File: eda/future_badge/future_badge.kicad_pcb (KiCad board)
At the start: 2 copper layers, 137.1 x 80 mm, 6 parts

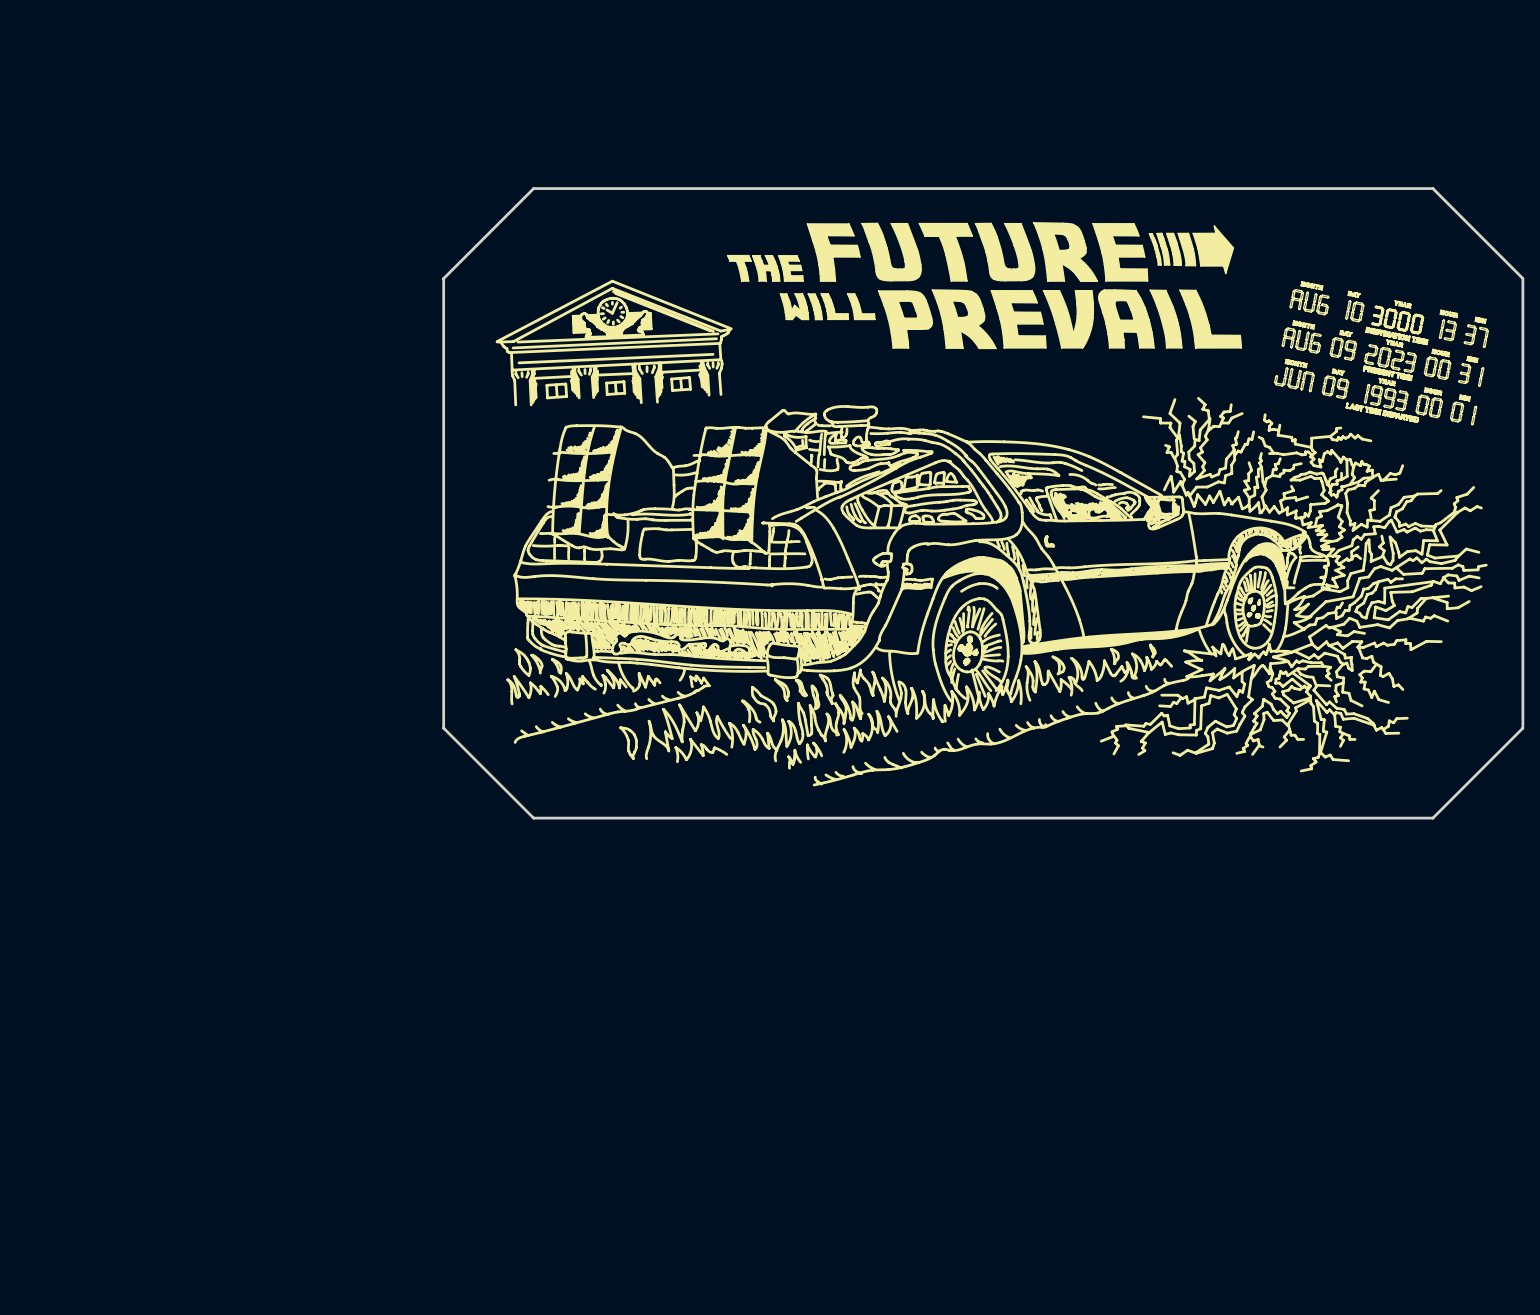
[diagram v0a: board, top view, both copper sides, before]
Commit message: PCB layout
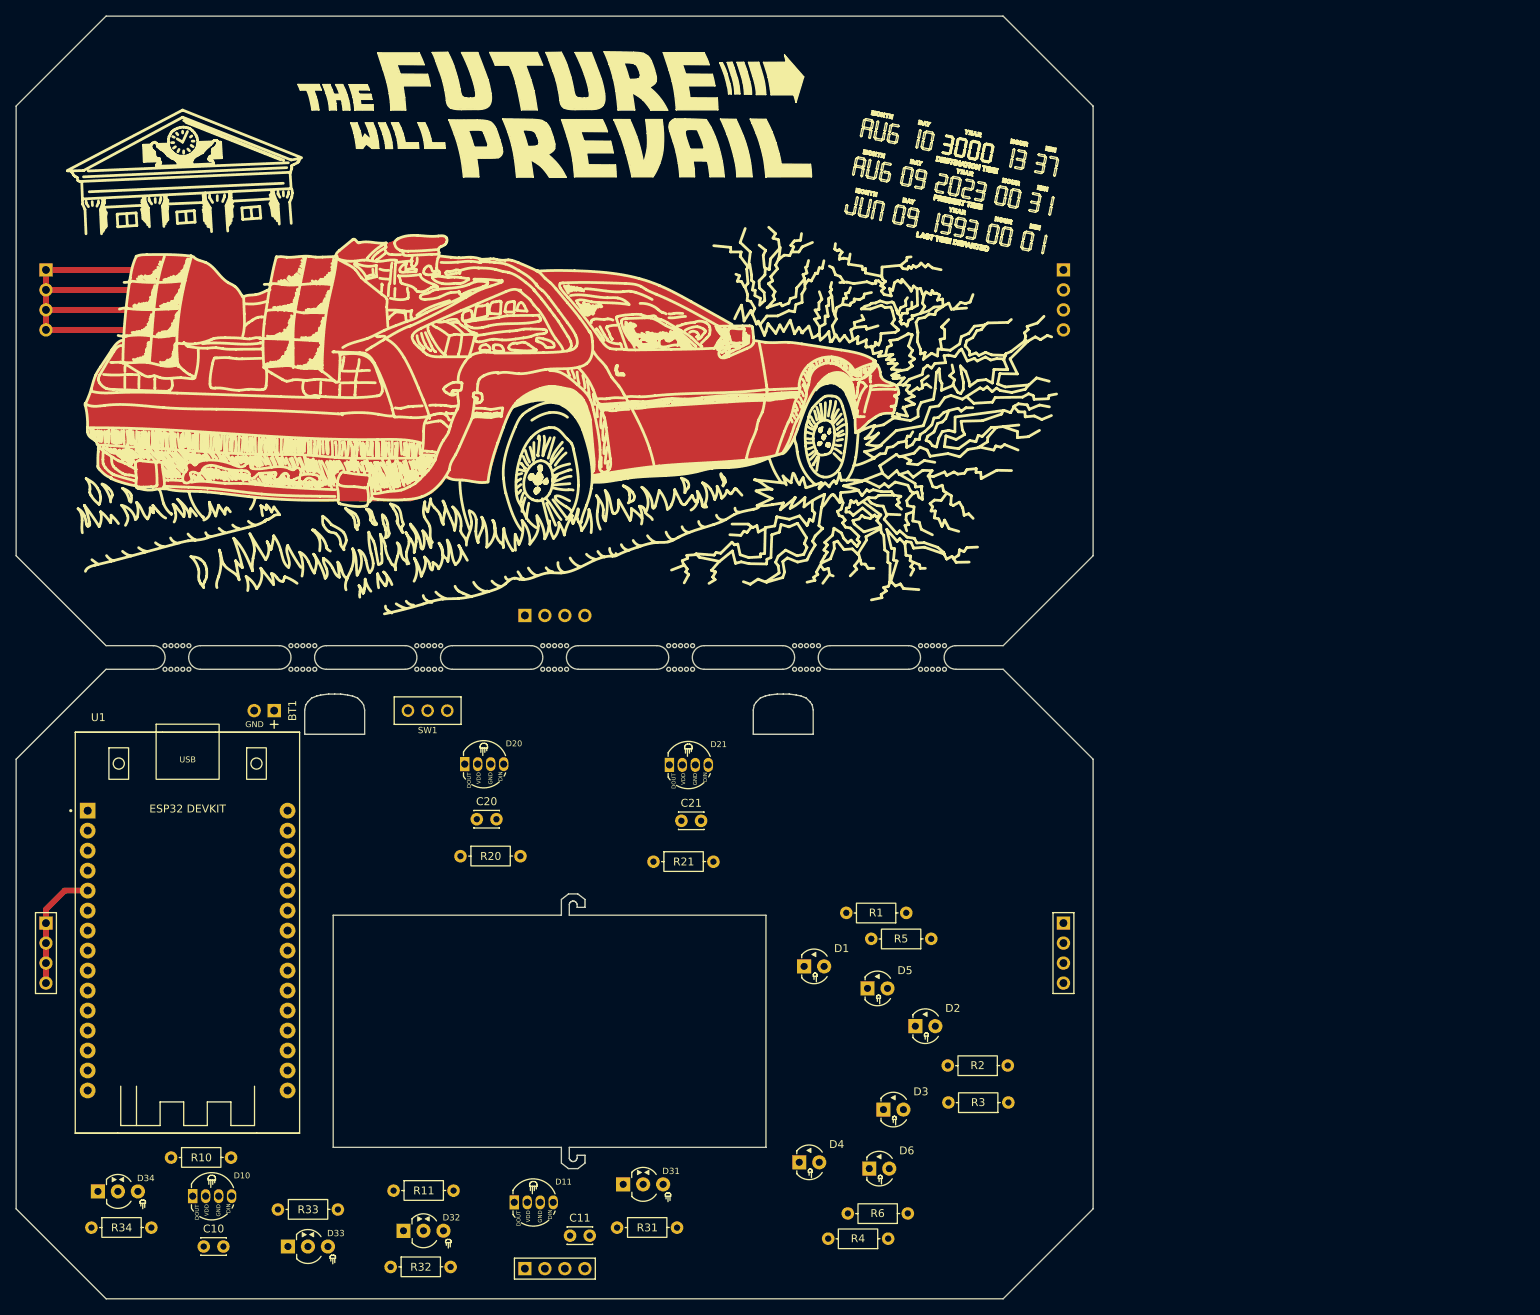
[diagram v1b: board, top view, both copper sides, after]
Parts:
- added BT1: Battery_9V, 0_local:Battery_Lead_Wire_Connector, F.Cu at (52.5, 106.0)
- added C10: 100nF, 0_local:C_Disc_D3.0mm_W2.0mm_P2.50mm, F.Cu at (43.5, 174.1)
- added C11: 100nF, 0_local:C_Disc_D3.0mm_W2.0mm_P2.50mm, F.Cu at (90.1, 172.7)
- added C20: 100nF, 0_local:C_Disc_D3.0mm_W2.0mm_P2.50mm, F.Cu at (78.2, 119.8)
- added C21: 100nF, 0_local:C_Disc_D3.0mm_W2.0mm_P2.50mm, F.Cu at (104.2, 120.0)
- added D1: LED_3mm, 0_local:LED_D3.0mm-2, F.Cu at (119.8, 138.5)
- added D10: LED_WS2812D_5mm, 0_local:LED_D5.0mm-4_WS2812D_front_new, F.Cu at (42.6, 167.7)
- added D11: LED_WS2812D_5mm, 0_local:LED_D5.0mm-4_WS2812D_front_new, F.Cu at (83.5, 168.5)
- added D2: LED_3mm, 0_local:LED_D3.0mm-2, F.Cu at (134.0, 146.1)
- added D20: LED_WS2812D_5mm, 0_local:LED_D5.0mm-4_WS2812D_front_new, F.Cu at (77.2, 112.8)
- added D21: LED_WS2812D_5mm, 0_local:LED_D5.0mm-4_WS2812D_front_new, F.Cu at (103.2, 112.9)
- added D3: LED_3mm, 0_local:LED_D3.0mm-2, F.Cu at (129.9, 156.7)
- added D31: YEL_RED_CC_3mm, 0_local:LED_D3.0mm-3-TwoColor, F.Cu at (96.8, 166.2)
- added D32: YEL_RED_CC_3mm, 0_local:LED_D3.0mm-3-TwoColor, F.Cu at (68.9, 172.1)
- added D33: YEL_RED_CC_3mm, 0_local:LED_D3.0mm-3-TwoColor, F.Cu at (54.2, 174.1)
- added D34: YEL_RED_CC_3mm, 0_local:LED_D3.0mm-3-TwoColor, F.Cu at (30.1, 167.1)
- added D4: LED_3mm, 0_local:LED_D3.0mm-2, F.Cu at (119.2, 163.4)
- added D5: LED_3mm, 0_local:LED_D3.0mm-2, F.Cu at (127.9, 141.3)
- added D6: LED_3mm, 0_local:LED_D3.0mm-2, F.Cu at (128.1, 164.2)
- added G***: 3000_Society_Logo_Back_2500dpi, 0_org_logos:3000_Society_Logo_Back_2500dpi, F.Cu at (65.5, 115.5)
- added G***: DHA_Logo_Back_1500dpi, 0_org_logos:DHA_Logo_Back_1500dpi, F.Cu at (134.0, 117.0)
- added G***: LOGO, 0_alt_bier:logo-alt_bier-500dpi-18x45mm-back, F.Cu at (41.5, 136.0)
- added G***: LOGO, 0_org_logos:DC214_Logo_v2_Back_1200dpi, F.Cu at (92.0, 112.0)
- added R1: 47R_6.3mm, 0_local:R_Axial_DIN0207_L6.3mm_D2.5mm_P7.62mm_Horizontal, F.Cu at (132.8, 131.7)
- added R10: 47R_6.3mm, 0_local:R_Axial_DIN0207_L6.3mm_D2.5mm_P7.62mm_Horizontal, F.Cu at (39.4, 162.8)
- added R11: 47R_6.3mm, 0_local:R_Axial_DIN0207_L6.3mm_D2.5mm_P7.62mm_Horizontal, F.Cu at (67.7, 167.0)
- added R2: 47R_6.3mm, 0_local:R_Axial_DIN0207_L6.3mm_D2.5mm_P7.62mm_Horizontal, F.Cu at (145.7, 151.1)
- added R20: 47R_6.3mm, 0_local:R_Axial_DIN0207_L6.3mm_D2.5mm_P7.62mm_Horizontal, F.Cu at (76.2, 124.5)
- added R21: 47R_6.3mm, 0_local:R_Axial_DIN0207_L6.3mm_D2.5mm_P7.62mm_Horizontal, F.Cu at (100.7, 125.2)
- added R3: 47R_6.3mm, 0_local:R_Axial_DIN0207_L6.3mm_D2.5mm_P7.62mm_Horizontal, F.Cu at (145.8, 155.8)
- added R31: 47R_6.3mm, 0_local:R_Axial_DIN0207_L6.3mm_D2.5mm_P7.62mm_Horizontal, F.Cu at (96.1, 171.7)
- added R32: 47R_6.3mm, 0_local:R_Axial_DIN0207_L6.3mm_D2.5mm_P7.62mm_Horizontal, F.Cu at (67.3, 176.7)
- added R33: 47R_6.3mm, 0_local:R_Axial_DIN0207_L6.3mm_D2.5mm_P7.62mm_Horizontal, F.Cu at (53.0, 169.4)
- added R34: 47R_6.3mm, 0_local:R_Axial_DIN0207_L6.3mm_D2.5mm_P7.62mm_Horizontal, F.Cu at (29.3, 171.7)
- added R4: 47R_6.3mm, 0_local:R_Axial_DIN0207_L6.3mm_D2.5mm_P7.62mm_Horizontal, F.Cu at (130.5, 173.1)
- added R5: 47R_6.3mm, 0_local:R_Axial_DIN0207_L6.3mm_D2.5mm_P7.62mm_Horizontal, F.Cu at (136.0, 135.0)
- added R6: 47R_6.3mm, 0_local:R_Axial_DIN0207_L6.3mm_D2.5mm_P7.62mm_Horizontal, F.Cu at (133.0, 169.9)
- added REF**: Conn_Pin_Header_Male_Vert_Front_1x04_Pitch2.54mm, 0_local:Conn_Pin_Header_Male_Vert_Front_1x04_Pitch2.54mm, F.Cu at (84.4, 176.9)
- added REF**: future_badge_userdrawing_title, 0_local:future_badge_userdrawing_title, F.Cu at (89.3, 129.1)
- added REF**: future_badge_frontcopper_delorean, 0_local:future_badge_frontcopper_delorean, F.Cu at (85.9, 59.5)
- added REF**: Battery_9V_silk_back, 0_local:Battery_9V_silk_back, F.Cu at (88.2, 63.7)
- added REF**: Conn_Pin_Header_Female_Vert_Back_1x04_Pitch2.54mm, 0_local:Conn_Pin_Header_Female_Vert_Back_1x04_Pitch2.54mm, F.Cu at (152.8, 50.0)
- added REF**: future_badge_userdrawing_flames, 0_local:future_badge_userdrawing_flames, F.Cu at (85.8, 138.2)
- added REF**: future_badge_frontmask_delorean, 0_local:future_badge_frontmask_delorean, F.Cu at (91.9, 54.4)
- added REF**: ESP32_DEVKIT_V1_silk_back, 0_local:ESP32_DEVKIT_V1_silk_back, F.Cu at (41.5, 51.2)
- added REF**: Conn_Pin_Header_Male_Vert_Front_1x04_Pitch2.54mm, 0_local:Conn_Pin_Header_Male_Vert_Front_1x04_Pitch2.54mm, F.Cu at (152.8, 133.0)
- added REF**: future_badge_backmask_flames, 0_local:future_badge_backmask_flames, F.Cu at (87.1, 52.4)
- added REF**: Conn_Pin_Header_Female_Vert_Back_1x04_Pitch2.54mm, 0_local:Conn_Pin_Header_Female_Vert_Back_1x04_Pitch2.54mm, F.Cu at (84.4, 93.9)
- added REF**: Conn_Pin_Header_Female_Vert_Back_1x04_Pitch2.54mm, 0_local:Conn_Pin_Header_Female_Vert_Back_1x04_Pitch2.54mm, F.Cu at (23.5, 50.0)
- added REF**: future_badge_backmask_title, 0_local:future_badge_backmask_title, F.Cu at (89.2, 51.2)
- added REF**: future_badge_userdrawing_lightning, 0_local:future_badge_userdrawing_lightning, F.Cu at (91.0, 132.5)
- added REF**: future_badge_frontmask_title, 0_local:future_badge_frontmask_title, F.Cu at (89.1, 46.2)
- added REF**: future_badge_backmask_lightning, 0_local:future_badge_backmask_lightning, F.Cu at (87.9, 47.1)
- added REF**: Conn_Pin_Header_Male_Vert_Front_1x04_Pitch2.54mm, 0_local:Conn_Pin_Header_Male_Vert_Front_1x04_Pitch2.54mm, F.Cu at (23.5, 133.0)
- added SW1: SPDT_SS12D00G, 0_local:SW_SPDT_Slide_SS12D00G-1P2T_3pin, F.Cu at (72.0, 106.0)
- added U1: ESP32-WROOM-32-DEVKIT, 0_local:ESP32_DEVKIT_V1, F.Cu at (41.5, 134.2)
- moved REF** 59.1 mm to (88.1, 100.2)
- moved REF** 58.8 mm to (90.7, 49.6)
- moved REF** 58.8 mm to (90.7, 37.2)
- moved REF** 58.8 mm to (92.5, 42.0)
- moved REF** 58.8 mm to (87.1, 50.9)
- moved REF** 58.8 mm to (85.5, 55.5)
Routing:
- net (no net): track 0.00 -> 50.3 mm
- net TOUCH: track 0.00 -> 15.7 mm
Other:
- board size 137.1 x 80 mm -> 136.9 x 163 mm

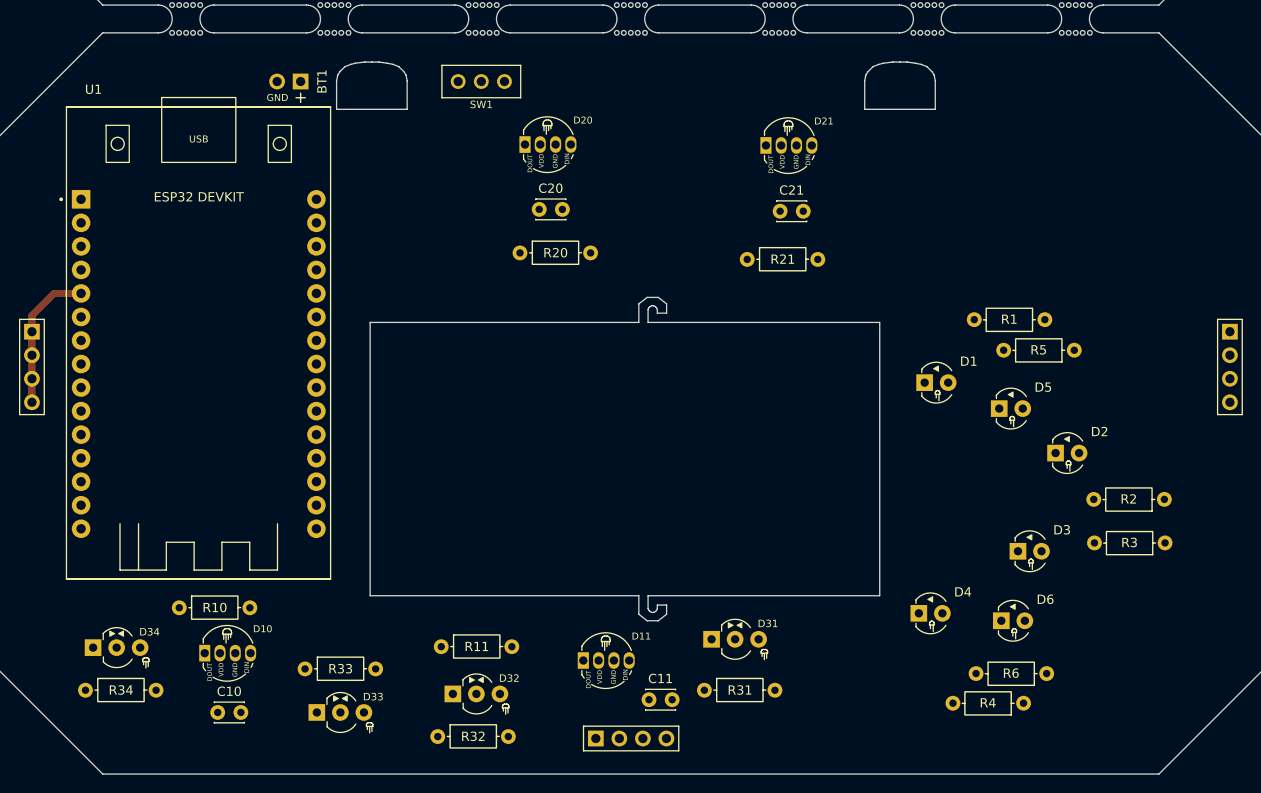
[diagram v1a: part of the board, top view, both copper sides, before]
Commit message: prototype ordered
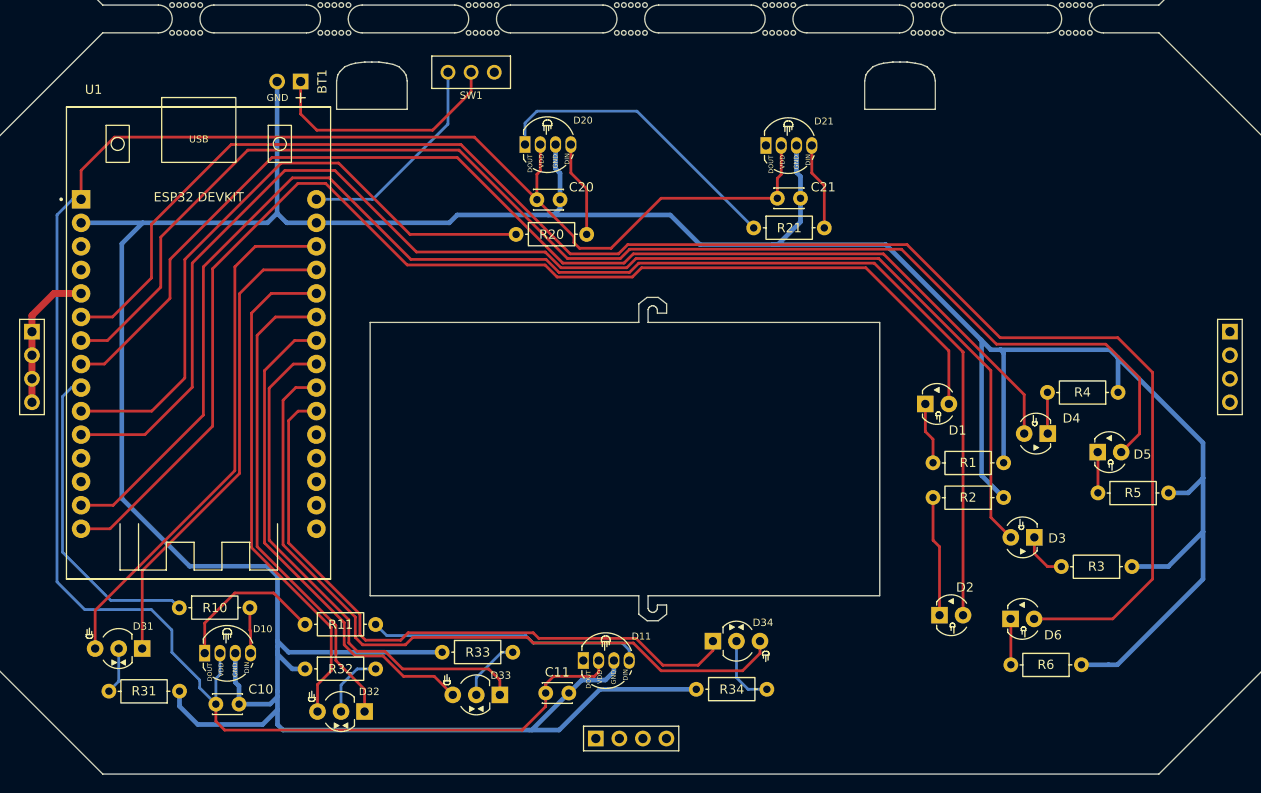
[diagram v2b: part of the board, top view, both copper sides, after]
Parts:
- added G***: LOGO, 0_org_logos:BSidesDFW_Logo_v2_Back_1800dpi, F.Cu at (70.2, 127.0)
- added G***: HackFtW_Logo_Back_5000dpi, 0_org_logos:HackFtW_Logo_Back_5000dpi, F.Cu at (118.3, 125.6)
- moved D34 66.9 mm to (97.0, 166.4)
- moved R34 65.9 mm to (95.2, 171.6)
- moved D31 61.5 mm to (35.4, 167.2), turned to 180 degrees
- moved R31 56.7 mm to (39.4, 171.8), turned to 180 degrees
- moved R4 35.1 mm to (140.7, 139.6)
- moved G*** 28.0 mm to (38.0, 110.3)
- moved D4 23.9 mm to (133.1, 144.0), turned to 180 degrees
- moved D2 21.5 mm to (121.5, 163.6)
- moved D33 19.8 mm to (74.0, 172.2), turned to 180 degrees
- moved R5 18.5 mm to (146.2, 150.4)
- moved R2 17.4 mm to (128.4, 150.9)
- moved R1 16.1 mm to (128.4, 147.2)
- moved R32 16.1 mm to (53.0, 169.4)
- moved R33 14.9 mm to (67.8, 167.6)
- moved R11 14.9 mm to (53.0, 164.6)
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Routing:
- net GND: track 0.00 -> 421.0 mm
- net +3.3V: track 0.00 -> 221.4 mm
- net LED06: track 0.00 -> 174.6 mm
- net LED02: track 0.00 -> 156.2 mm
- net LED03: track 0.00 -> 146.5 mm
- net LED05: track 0.00 -> 145.8 mm
- net LED01: track 0.00 -> 133.1 mm
- net LED04: track 0.00 -> 129.1 mm
- net LED34B: track 0.00 -> 80.9 mm
- net LED34A: track 0.00 -> 71.5 mm
- net NEO2: track 0.00 -> 68.7 mm
- net LED31B: track 0.00 -> 57.2 mm
- net LED33A: track 0.00 -> 56.8 mm
- net LED32B: track 0.00 -> 55.1 mm
- net LED33B: track 0.00 -> 54.1 mm
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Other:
- board text added: "Badge Details = https://futurebadge.altbier.us/"
